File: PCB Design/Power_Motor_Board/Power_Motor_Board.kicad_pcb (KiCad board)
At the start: 2 copper layers, 100 x 87.1 mm, 38 parts, among them IC1 DRV8251ADDAR, IC2 AP63205WU-7, IC3 DRV8251ADDAR, IC4 AP63205WU-7, J1 691137710002, J2 691137710002, J2A1 SSW-119-01-T-D, J3 691137710002, J4 Conn_01x06

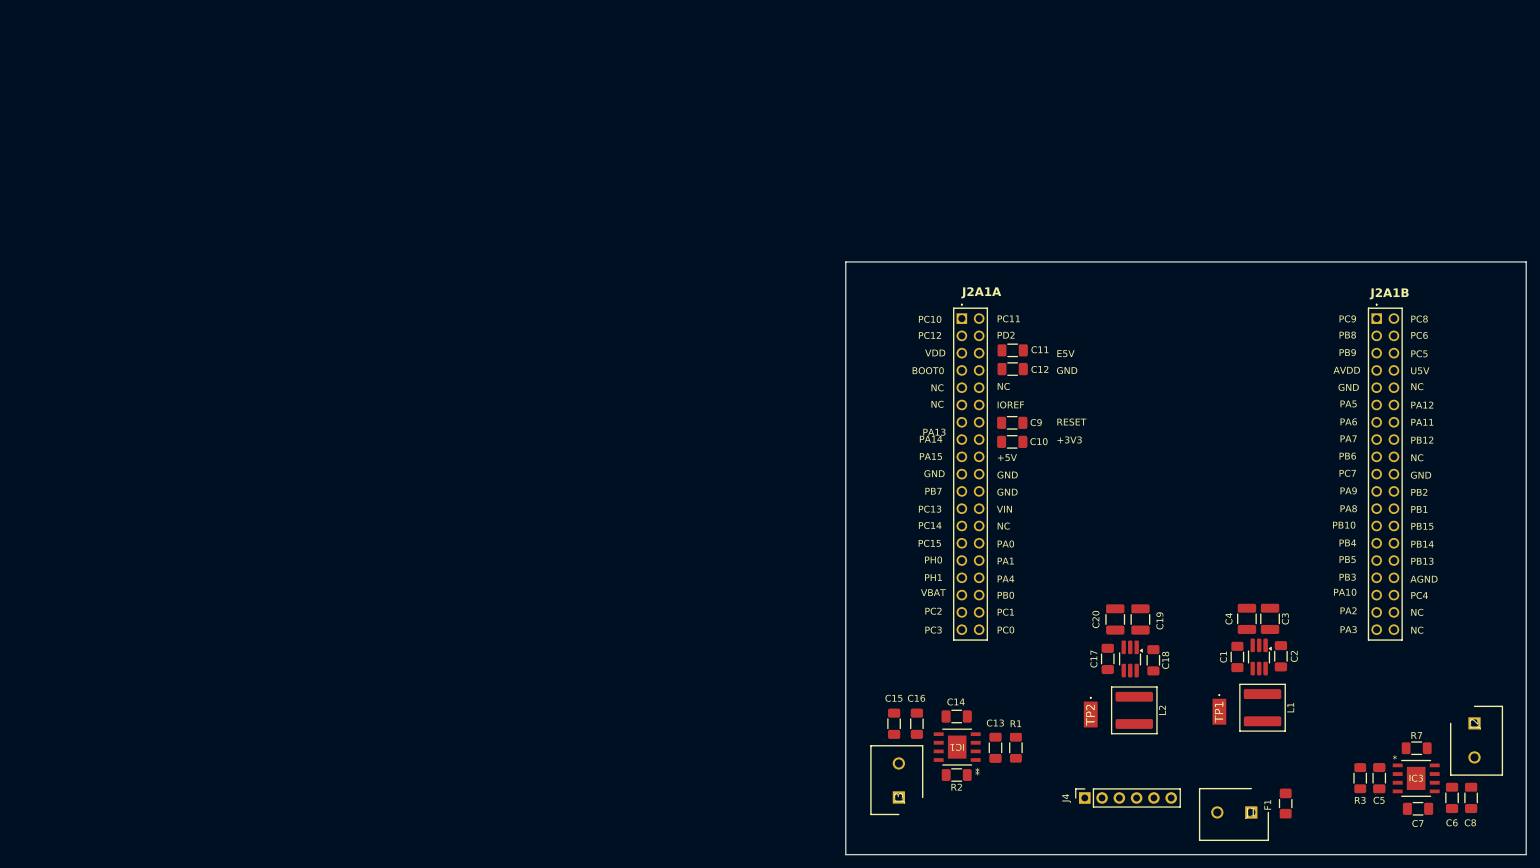
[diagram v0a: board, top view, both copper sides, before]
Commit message: First Revision of Power_Motor PCB
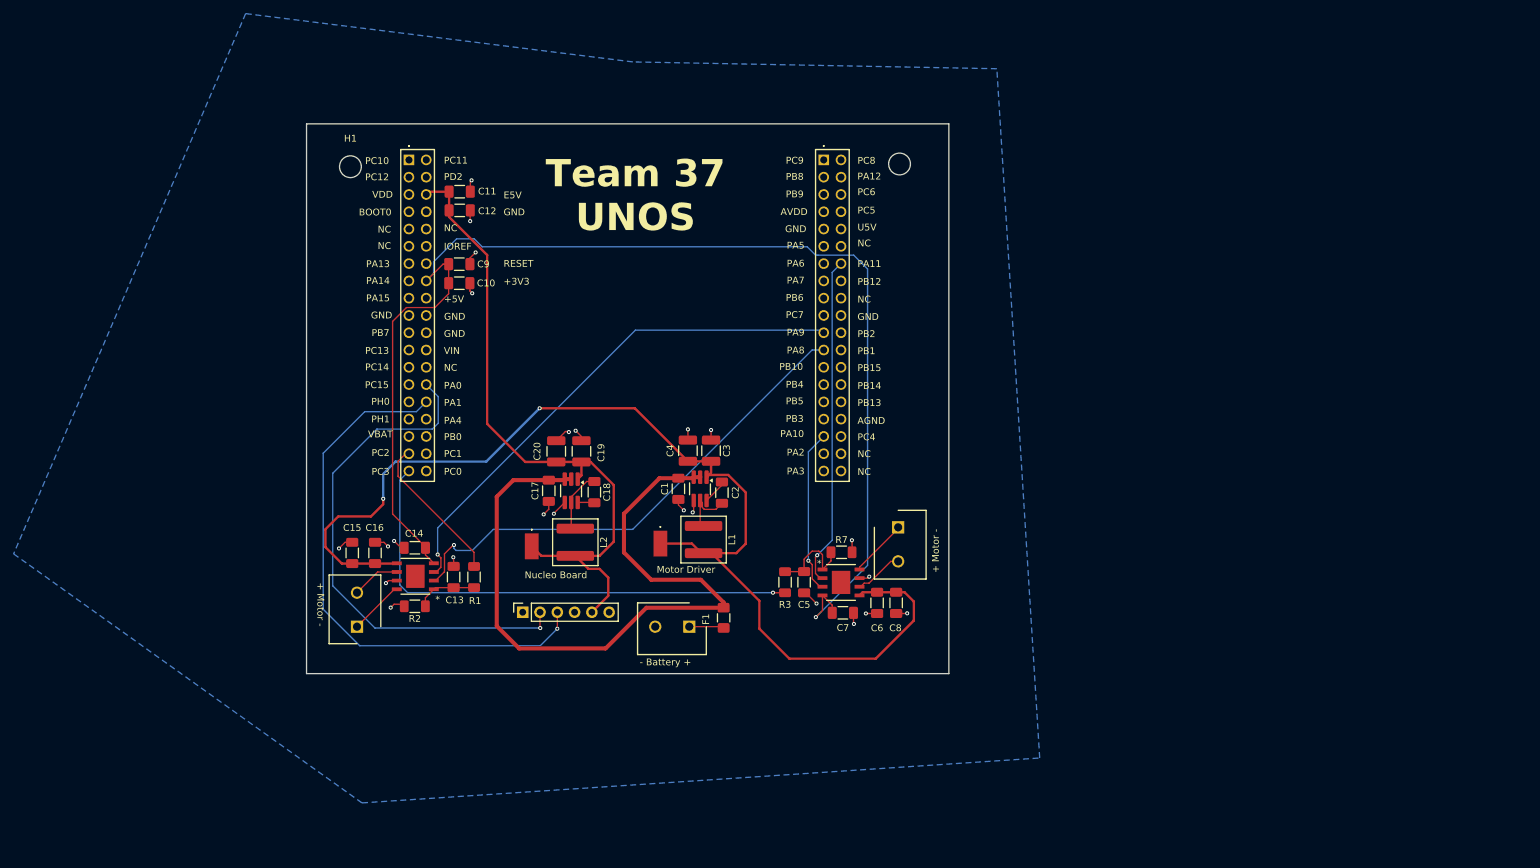
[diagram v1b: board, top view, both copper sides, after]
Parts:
- added G***: LOGO, LOGO, F.Cu at (152.3, 52.3)
- added H1: MountingHole, MountingHole:MountingHole_3.2mm_M3, F.Cu at (110.8, 48.7)
- added H2: MountingHole, MountingHole:MountingHole_3.2mm_M3, F.Cu at (191.5, 48.3)
- moved J2 89.5 mm to (191.3, 101.7)
- moved C5 89.3 mm to (177.5, 109.8)
- moved C7 89.3 mm to (183.2, 114.3)
- moved IC3 89.3 mm to (182.9, 109.8)
- moved R3 89.3 mm to (174.7, 109.8)
- moved R7 89.3 mm to (183.0, 105.4)
- moved C6 89.2 mm to (188.2, 112.8)
- moved C8 89.2 mm to (191.0, 112.8)
- moved F1 87.0 mm to (165.7, 115.0)
- moved J1 87.0 mm to (160.6, 116.3)
- moved J4 87.0 mm to (136.1, 114.2)
- moved C1 85.8 mm to (159.0, 96.0)
- moved C17 85.8 mm to (139.9, 96.3)
- moved C18 85.8 mm to (146.7, 96.5)
- moved C19 85.8 mm to (144.8, 90.5)
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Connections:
- C15 pad 1: Vbatt -> 5V
- C16 pad 1: Vbatt -> 5V
- C3 pad 2: +5V -> 5V
- C4 pad 2: +5V -> 5V
- C6 pad 1: Vbatt -> 5V
- C8 pad 1: Vbatt -> 5V
- IC1 pad 5: Vbatt -> 5V
- IC1 pad 6: /+OUT -> /+OUT_1
- IC1 pad 8: /-OUT -> /-OUT_1
- IC2 pad 1: +5V -> 5V
- IC3 pad 5: Vbatt -> 5V
- IC3 pad 6: /+OUT -> /+OUT_2
- IC3 pad 8: /-OUT -> /-OUT_2
- J2 pad 1: /-OUT -> /-OUT_2
- J2 pad 2: /+OUT -> /+OUT_2
- J3 pad 1: /-OUT -> /-OUT_1
- J3 pad 2: /+OUT -> /+OUT_1
- L1 pad 2: +5V -> 5V
- TP1 pad 1: +5V -> 5V
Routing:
- net +3V3: track 0.00 -> 188.0 mm, vias 0 -> 1
- net 5V: track 0.00 -> 168.4 mm, vias 0 -> 2
- net +Vbatt: track 0.00 -> 105.8 mm
- net +5V: track 0.00 -> 99.1 mm
- net /BT_TX: track 0.00 -> 81.3 mm, vias 0 -> 1
- net /BT_RX: track 0.00 -> 76.9 mm, vias 0 -> 1
- net /IN1_MTR1: track 0.00 -> 76.2 mm, vias 0 -> 1
- net /I_MTR2: track 0.00 -> 74.4 mm, vias 0 -> 1
- net /IN2-MTR1: track 0.00 -> 73.8 mm, vias 0 -> 1
- net /IN2_MTR2: track 0.00 -> 48.4 mm, vias 0 -> 1
- net GND: track 0.00 -> 45.3 mm, vias 0 -> 24
- net /IN1_MTR2: track 0.00 -> 24.1 mm, vias 0 -> 1
- net /I_MTR1: track 0.00 -> 22.1 mm
- net Net-(IC3-IPROPI): track 0.00 -> 13.3 mm
- net Net-(IC4-SW): track 0.00 -> 9.25 mm
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- added copper zone on B.Cu, net GND
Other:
- board size 100 x 87.1 mm -> 94.4 x 80.8 mm
- board text added: "+ Motor -"
- board text added: "- Battery +"
- board text added: "Motor Driver"
- board text added: "Nucleo Board"
- board text added: "Team 37 UNOS"
- board text added: "amazingamy"
- board text added: "freddy fazbear"
- board text added: "jujuthepoopoo"
- board text added: "lean masheen"
- board text added: "whatdahaleeberry"
